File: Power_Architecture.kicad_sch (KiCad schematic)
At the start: 0 parts

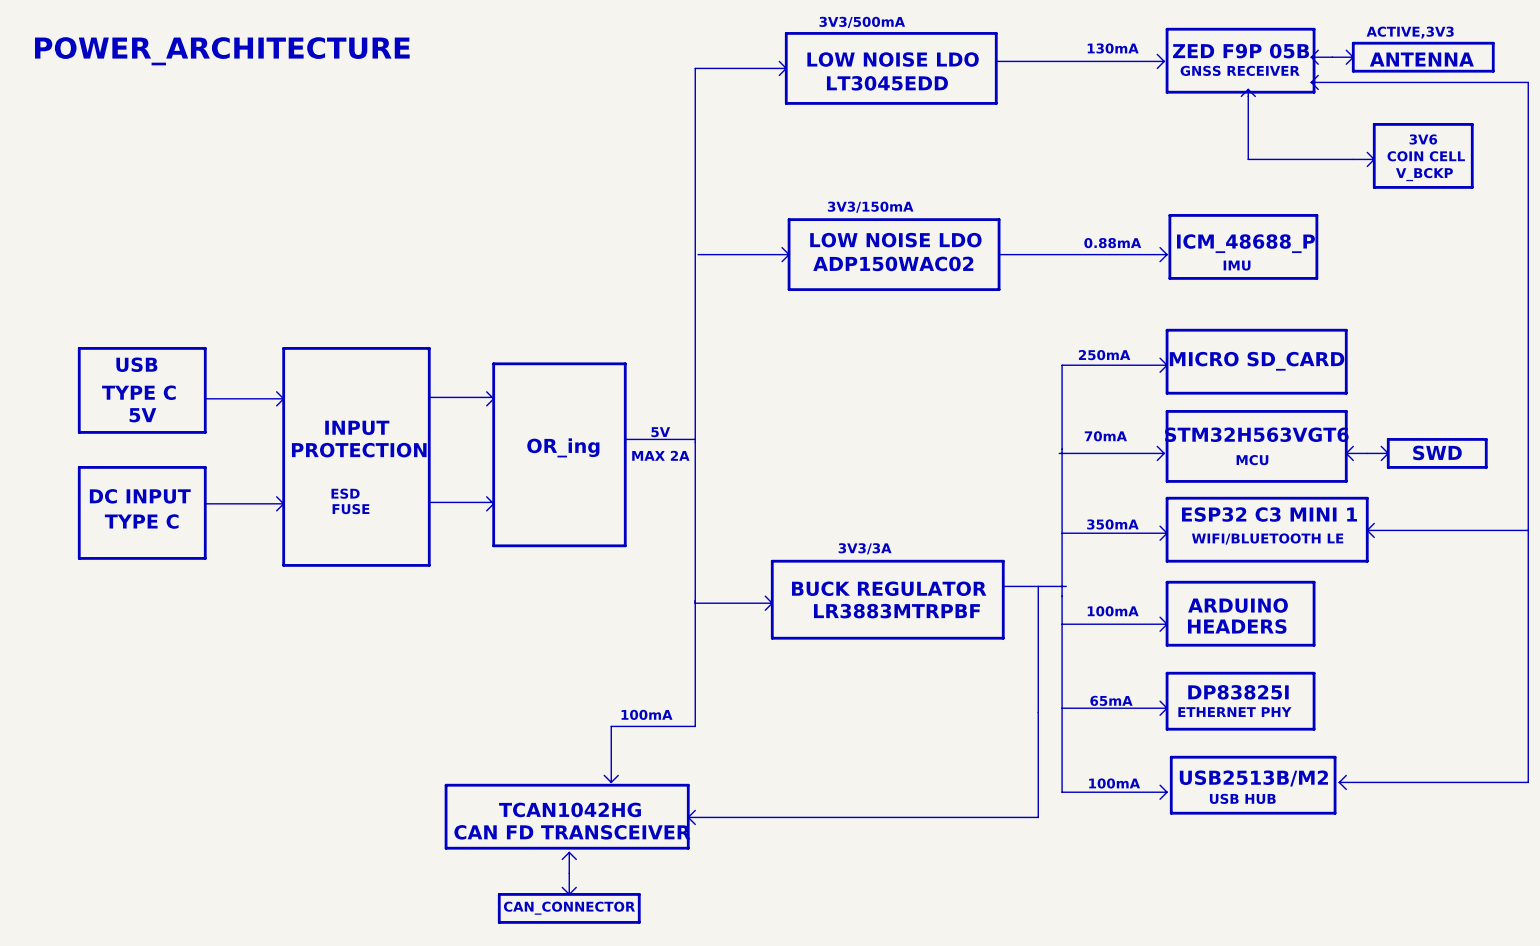
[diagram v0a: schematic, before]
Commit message: new
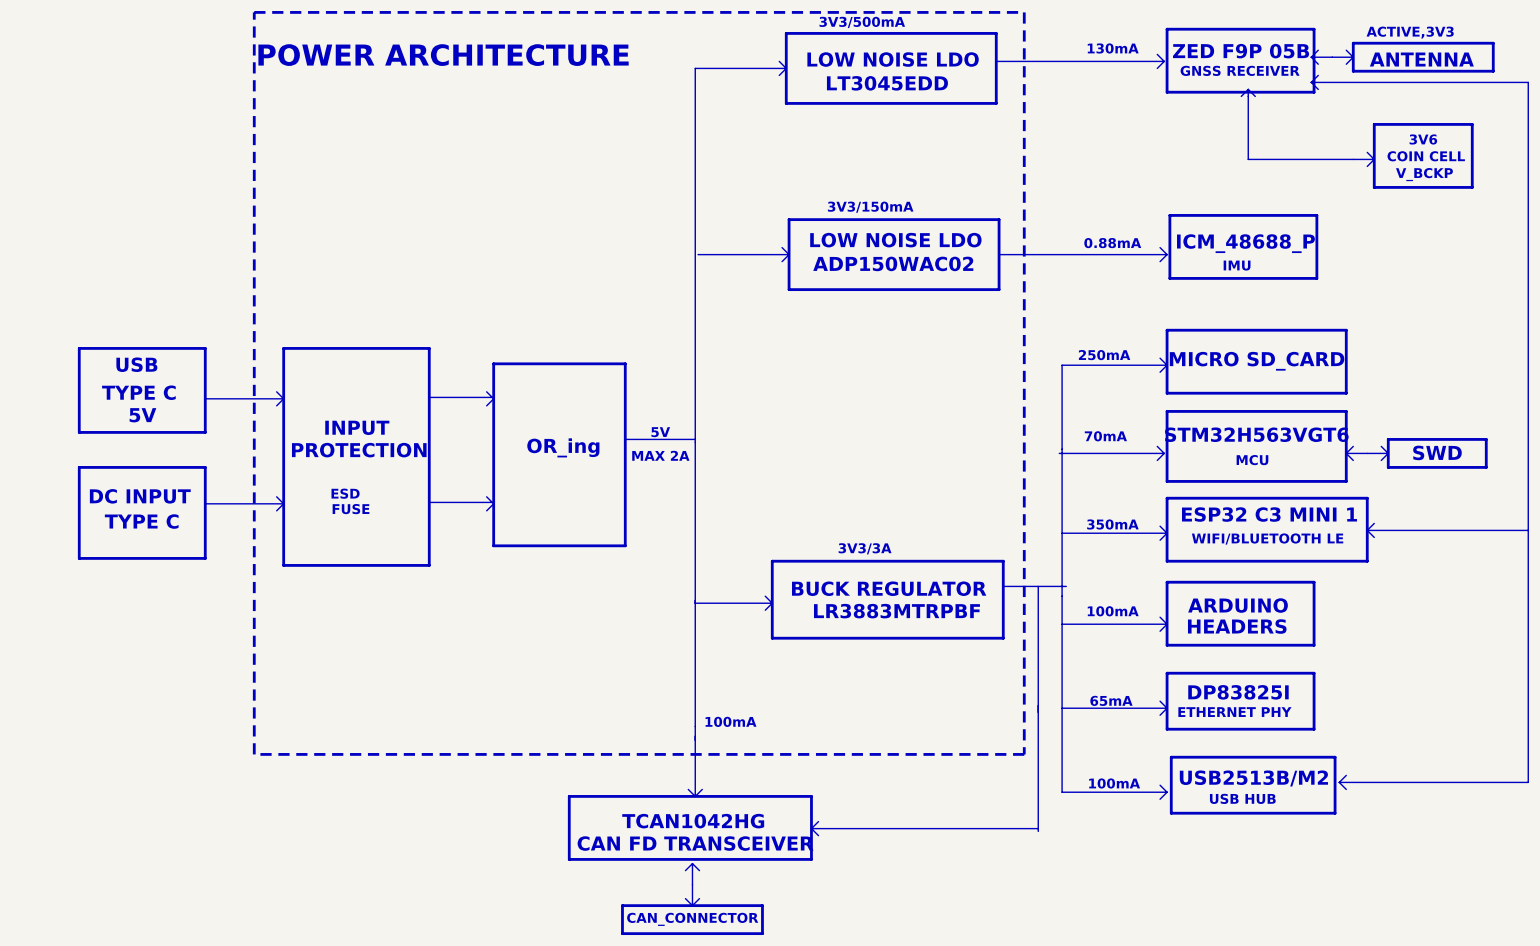
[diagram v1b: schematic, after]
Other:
- note added: "POWER ARCHITECTURE"
- note removed: "POWER_ARCHITECTURE"
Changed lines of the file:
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@@
 	(polyline
 		(pts
-			(xy 132.08 142.24) (xy 116.84 142.24)
+			(xy 132.08 142.24) (xy 132.08 144.78)
 		)
 		(stroke
@@
 	(polyline
 		(pts
-			(xy 194.31 139.7) (xy 194.31 158.75)
+			(xy 194.31 138.43) (xy 194.31 161.29)
 		)
 		(stroke
@@
 	(polyline
 		(pts
-			(xy 132.08 160.02) (xy 130.81 158.75)
+			(xy 154.432 162.052) (xy 153.162 160.782)
 		)
 		(stroke
@@
 	(polyline
 		(pts
-			(xy 110.49 166.37) (xy 109.22 165.1)
+			(xy 132.842 168.402) (xy 131.572 167.132)
 		)
 		(stroke
@@
 	(polyline
 		(pts
-			(xy 109.22 172.72) (xy 109.22 168.91)
+			(xy 131.572 174.752) (xy 131.572 170.942)
 		)
 		(stroke
@@
 	(polyline
 		(pts
-			(xy 107.95 171.45) (xy 109.22 172.72)
+			(xy 130.302 173.482) (xy 131.572 174.752)
 		)
 		(stroke
@@
 	(polyline
 		(pts
-			(xy 118.11 151.13) (xy 116.84 152.4)
+			(xy 133.35 153.67) (xy 132.08 154.94)
 		)
 		(stroke
@@
 	(polyline
 		(pts
-			(xy 132.08 157.48) (xy 130.81 158.75)
-		)
-		(stroke
-			(width 0.254)
-			(type default)
-			(color 0 0 0 1)
-		)
-	)
-	(polyline
-		(pts
-			(xy 115.57 151.13) (xy 116.84 152.4)
+			(xy 154.432 159.512) (xy 153.162 160.782)
+		)
+		(stroke
+			(width 0.254)
+			(type default)
+			(color 0 0 0 1)
+		)
+	)
+	(polyline
+		(pts
+			(xy 130.81 153.67) (xy 132.08 154.94)
 		)
 		(stroke
@@
 	(polyline
 		(pts
-			(xy 109.22 168.91) (xy 109.22 165.1)
-		)
-		(stroke
-			(width 0.254)
-			(type default)
-			(color 0 0 0 1)
-		)
-	)
-	(polyline
-		(pts
-			(xy 130.81 158.75) (xy 194.31 158.75)
+			(xy 131.572 170.942) (xy 131.572 167.132)
+		)
+		(stroke
+			(width 0.254)
+			(type default)
+			(color 0 0 0 1)
+		)
+	)
+	(polyline
+		(pts
+			(xy 153.162 160.782) (xy 194.31 160.782)
 		)
 		(stroke
@@
 	(polyline
 		(pts
-			(xy 107.95 166.37) (xy 109.22 165.1)
+			(xy 130.302 168.402) (xy 131.572 167.132)
 		)
 		(stroke
@@
 	(polyline
 		(pts
-			(xy 116.84 142.24) (xy 116.84 152.4)
+			(xy 132.08 144.018) (xy 132.08 154.94)
 		)
 		(stroke
@@
 	(polyline
 		(pts
-			(xy 110.49 171.45) (xy 109.22 172.72)
+			(xy 132.842 173.482) (xy 131.572 174.752)
 		)
 		(stroke
@@
 	)
 	(rectangle
-		(start 96.52 172.72)
-		(end 121.92 177.8)
+		(start 118.872 174.752)
+		(end 144.272 179.832)
 		(stroke
 			(width 0.508)
@@
 	)
 	(rectangle
+		(start 52.07 12.7)
+		(end 191.77 147.32)
+		(stroke
+			(width 0.508)
+			(type dot)
+			(color 72 72 72 1)
+		)
+		(fill
+			(type none)
+		)
+	)
+	(rectangle
 		(start 95.504 76.454)
 		(end 119.38 109.474)
@@
 	)
 	(rectangle
-		(start 86.868 152.908)
-		(end 130.81 164.338)
+		(start 109.22 154.94)
+		(end 153.162 166.37)
 		(stroke
 			(width 0.508)
@@
 	(text "100mA"
 		(exclude_from_sim no)
-		(at 123.19 140.462 0)
+		(at 138.43 141.732 0)
 		(effects
 			(font
@@
 		)
 	)
-	(text "POWER_ARCHITECTURE"
-		(exclude_from_sim no)
-		(at 46.228 19.558 0)
+	(text "POWER ARCHITECTURE"
+		(exclude_from_sim no)
+		(at 86.36 20.828 0)
 		(effects
 			(font
@@
 	(text "CAN FD TRANSCEIVER"
 		(exclude_from_sim no)
-		(at 109.728 161.798 0)
+		(at 132.08 163.83 0)
 		(effects
 			(font
@@
 	(text "CAN_CONNECTOR"
 		(exclude_from_sim no)
-		(at 109.22 175.26 0)
+		(at 131.572 177.292 0)
 		(effects
 			(font
@@
 	(text "TCAN1042HG"
 		(exclude_from_sim no)
-		(at 109.474 157.734 0)
-		(effects
-			(font
+		(at 131.826 159.766 0)
+		(effects
+			(font
